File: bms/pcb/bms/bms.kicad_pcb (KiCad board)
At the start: 2 copper layers, 52.7 x 86.2 mm, 40 parts, among them IC1 NCV8402ASTT1G, IC2 NCV8402ASTT1G, IC3 MCP2515-I_ST, IC4 MCP2515-I_ST, IC5 MCP2515-I_ST, IC6 SN65HVD230, IC7 SN65HVD230, IC8 SN65HVD230, IC9 TPS62160DGKR, J1 power, J2 MAIN CAN, J3 BATT1 CAN, J4 BATT2 CAN, J5 INPUTS, J6 INPUTS, J7 M22-2510346, U8 Pico

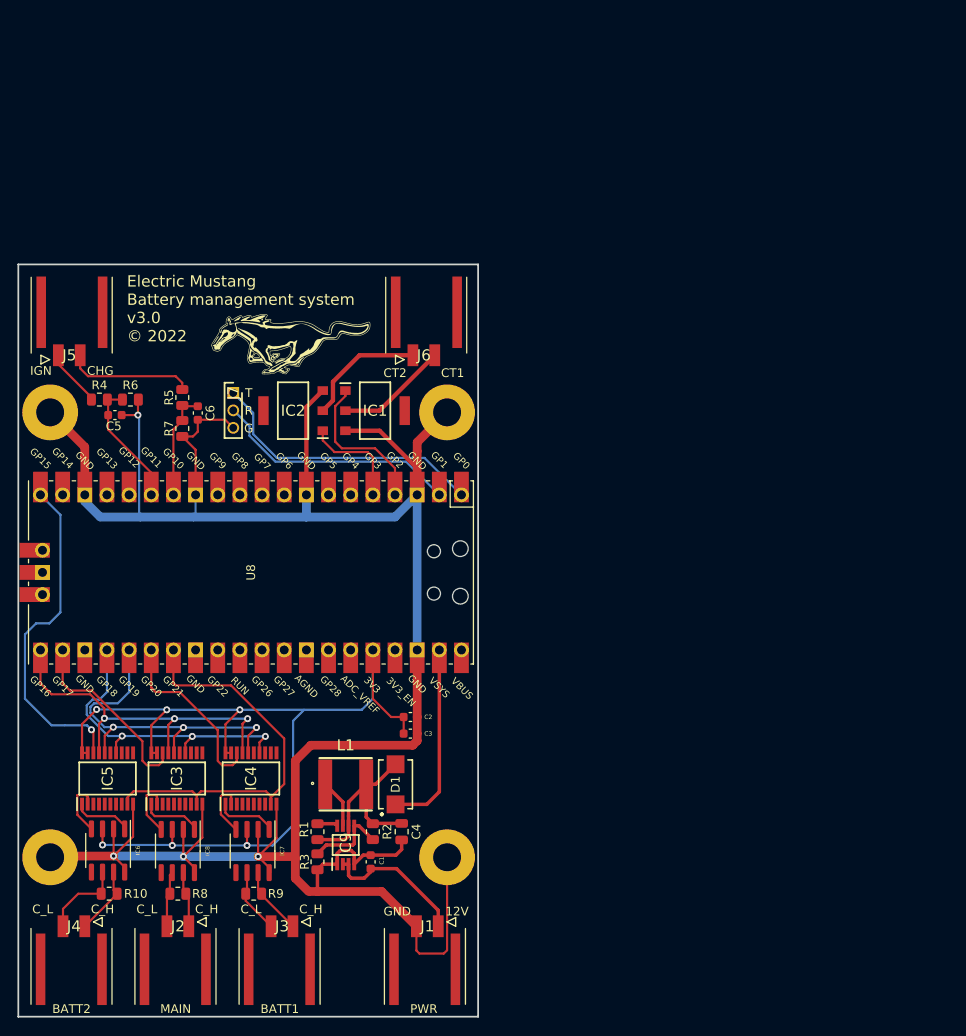
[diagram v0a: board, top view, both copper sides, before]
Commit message: BMS pcb v4
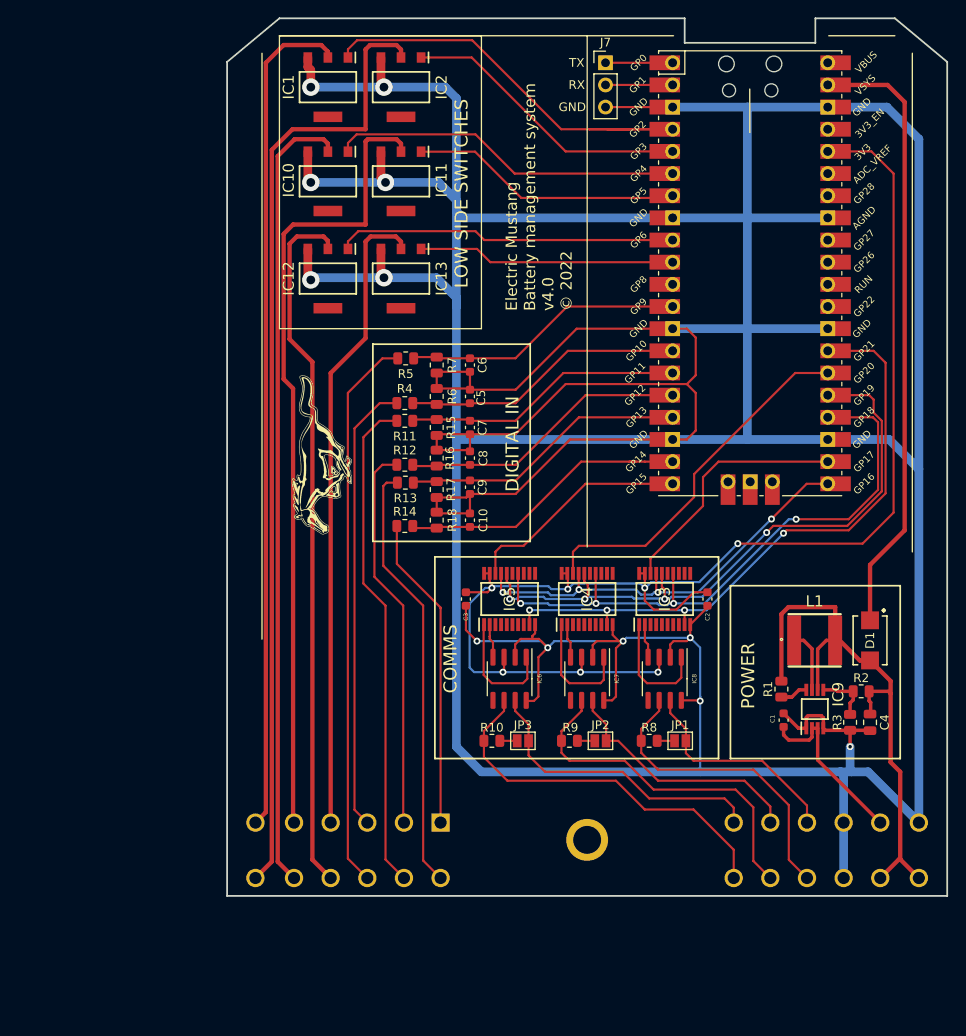
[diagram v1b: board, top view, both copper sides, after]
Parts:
- removed H1, H2, H3, H4: MountingHole, MountingHole:MountingHole_3.2mm_M3_Pad
- removed J1: power, Connector:105430YY02
- removed J2: MAIN CAN, Connector:105430YY02
- removed J3: BATT1 CAN, Connector:105430YY02
- removed J4: BATT2 CAN, Connector:105430YY02
- removed J5, J6: INPUTS, Connector:105430YY02
- added C10: 1uF, Capacitor_SMD:C_0603_1608Metric, F.Cu at (121.6, 111.4)
- added C7: 1uF, Capacitor_SMD:C_0603_1608Metric, F.Cu at (121.6, 100.7)
- added C8: 1uF, Capacitor_SMD:C_0603_1608Metric, F.Cu at (121.6, 104.2)
- added C9: 1uF, Capacitor_SMD:C_0603_1608Metric, F.Cu at (121.6, 107.6)
- added IC10: NCV8402ASTT1G, Symbol:SOT230P700X175-4N, F.Cu at (105.3, 72.5)
- added IC11: NCV8402ASTT1G, Symbol:SOT230P700X175-4N, F.Cu at (113.7, 72.5)
- added IC12: NCV8402ASTT1G, Symbol:SOT230P700X175-4N, F.Cu at (105.3, 83.7)
- added IC13: NCV8402ASTT1G, Symbol:SOT230P700X175-4N, F.Cu at (113.7, 83.7)
- added JP1: SolderJumper_2_Open, Jumper:SolderJumper-2_P1.3mm_Open_Pad1.0x1.5mm, F.Cu at (145.7, 136.7)
- added JP2: SolderJumper_2_Open, Jumper:SolderJumper-2_P1.3mm_Open_Pad1.0x1.5mm, F.Cu at (136.6, 136.7)
- added JP3: SolderJumper_2_Open, Jumper:SolderJumper-2_P1.3mm_Open_Pad1.0x1.5mm, F.Cu at (127.7, 136.7)
- added R11: 4k7, Resistor_SMD:R_0805_2012Metric, F.Cu at (114.2, 100.0)
- added R12: 4k7, Resistor_SMD:R_0805_2012Metric, F.Cu at (114.2, 105.0)
- added R13: 4k7, Resistor_SMD:R_0805_2012Metric, F.Cu at (114.2, 107.1)
- added R14: 4k7, Resistor_SMD:R_0805_2012Metric, F.Cu at (114.2, 112.0)
- added R15: 1k5, Resistor_SMD:R_0805_2012Metric, F.Cu at (117.8, 100.7)
- added R16: 1k5, Resistor_SMD:R_0805_2012Metric, F.Cu at (117.8, 104.2)
- added R17: 1k5, Resistor_SMD:R_0805_2012Metric, F.Cu at (117.8, 107.8)
- added R18: 1k5, Resistor_SMD:R_0805_2012Metric, F.Cu at (117.8, 111.4)
- added X1: ATM13-12PB-12PC-BM03, Connector:ATM1312PB12PCBM03, F.Cu at (118.3, 146.0)
- J7: footprint Connector:HDRV3W50P0X200_1X3_600X200X525P -> Connector_PinHeader_2.54mm:PinHeader_1x03_P2.54mm_Vertical
- moved U8 66.7 mm to (153.7, 83.1), turned to 0 degrees
- moved R3 63.1 mm to (165.2, 134.5)
- moved IC3 59.6 mm to (143.9, 120.4)
- moved IC8 59.2 mm to (143.9, 129.5)
- moved R2 58.2 mm to (166.5, 131.0), turned to 180 degrees
- moved J7 57.0 mm to (137.2, 58.9), turned to 0 degrees
- moved D1 56.8 mm to (167.5, 125.1), turned to -90 degrees
- moved R8 56.8 mm to (142.2, 136.7)
- moved L1 56.2 mm to (161.1, 125.1)
- moved IC9 56.0 mm to (161.2, 133.0)
- moved R1 55.6 mm to (157.3, 130.7), turned to -90 degrees
- moved C4 55.1 mm to (167.5, 134.5)
- moved IC5 50.5 mm to (126.2, 120.4)
- moved IC6 50.1 mm to (126.2, 129.5)
- moved C1 50.0 mm to (157.6, 134.3)
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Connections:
- net BATT_1_CONTACTOR_SIGNAL renamed BATT_1_INHIBIT_SIGNAL
- net BATT_2_CONTACTOR_SIGNAL renamed BATT_2_INHIBIT_SIGNAL
- IC1 pad 2: BATT_1_CONTACTOR_GND -> BATT_1_INHIBIT
- IC2 pad 2: BATT_2_CONTACTOR_GND -> BATT_2_INHIBIT
- R10 pad 2: BATT_2_CAN_H -> Net-(JP3-Pad1)
- R8 pad 2: MAIN_CAN_H -> Net-(JP1-Pad1)
- R9 pad 2: BATT_1_CAN_H -> Net-(JP2-Pad1)
- U8 pad 10: unconnected-(U8-Pad10) -> OUT_4_SIGNAL
- U8 pad 12: unconnected-(U8-Pad12) -> CHARGE_ENABLE_IN_SIGNAL
- U8 pad 14: CHARGE_ENABLE_IN_SIGNAL -> IGNITION_ON_IN_SIGNAL
- U8 pad 15: IGNITION_ON_IN_SIGNAL -> IN_1_SIGNAL
- U8 pad 16: unconnected-(U8-Pad16) -> IN_2_SIGNAL
- U8 pad 17: unconnected-(U8-Pad17) -> IN_3_SIGNAL
- U8 pad 19: unconnected-(U8-Pad19) -> IN_4_SIGNAL
- U8 pad 23: unconnected-(U8-Pad23) -> GND
- U8 pad 28: unconnected-(U8-Pad28) -> GND
- U8 pad 33: unconnected-(U8-Pad33) -> GND
- U8 pad 6: unconnected-(U8-Pad6) -> OUT_1_SIGNAL
- U8 pad 7: unconnected-(U8-Pad7) -> OUT_2_SIGNAL
- U8 pad 9: unconnected-(U8-Pad9) -> OUT_3_SIGNAL
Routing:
- net GND: track 296.5 -> 726.4 mm, vias 4 -> 12
- net BATT_2_INHIBIT: track 0.00 -> 110.5 mm
- net BATT_1_INHIBIT: track 0.00 -> 96.5 mm
- net OUT_2: track 0.00 -> 92.6 mm
- net OUT_1: track 0.00 -> 91.2 mm
- net OUT_3: track 0.00 -> 80.5 mm
- net OUT_4: track 0.00 -> 73.6 mm
- net IN_1: track 0.00 -> 57.1 mm
- net IN_3: track 0.00 -> 49.4 mm
- net CHARGE_ENABLE_IN: track 14.7 -> 63.9 mm
- net Net-(D1-Pad1): track 21.9 -> 70.7 mm
- net IGNITION_ON_IN: track 6.65 -> 51.9 mm
- net 3V: track 110.7 -> 155.8 mm, vias 6 -> 7
- net IN_2: track 0.00 -> 44.5 mm
- net 5V: track 23.0 -> 65.8 mm
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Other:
- board size 52.7 x 86.2 mm -> 82.6 x 100.6 mm
- board text added: "COMMS"
- board text added: "DIGITAL IN"
- board text added: "Electric Mustang Battery management system v4.0 © 2022"
- board text added: "LOW SIDE SWITCHES"
- board text added: "POWER"
- board text added: "RX"
- board text added: "TX"
- board text removed: "12V"
- board text removed: "BATT1"
- board text removed: "BATT2"
- board text removed: "CHG"
- board text removed: "CT1"
- board text removed: "CT2"
- board text removed: "C_H"
- board text removed: "C_L"
- board text removed: "Electric Mustang Battery management system v3.0 © 2022"
- board text removed: "G"
- board text removed: "IGN"
- board text removed: "MAIN"
- board text removed: "PWR"
- board text removed: "R"
- board text removed: "T"
